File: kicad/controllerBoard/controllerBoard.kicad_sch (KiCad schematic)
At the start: 19 parts, among them J1 Conn_02x20_Top_Bottom, J2 Conn_02x20_Top_Bottom, Q1 WTM30N02VD, U1 LM3478MA

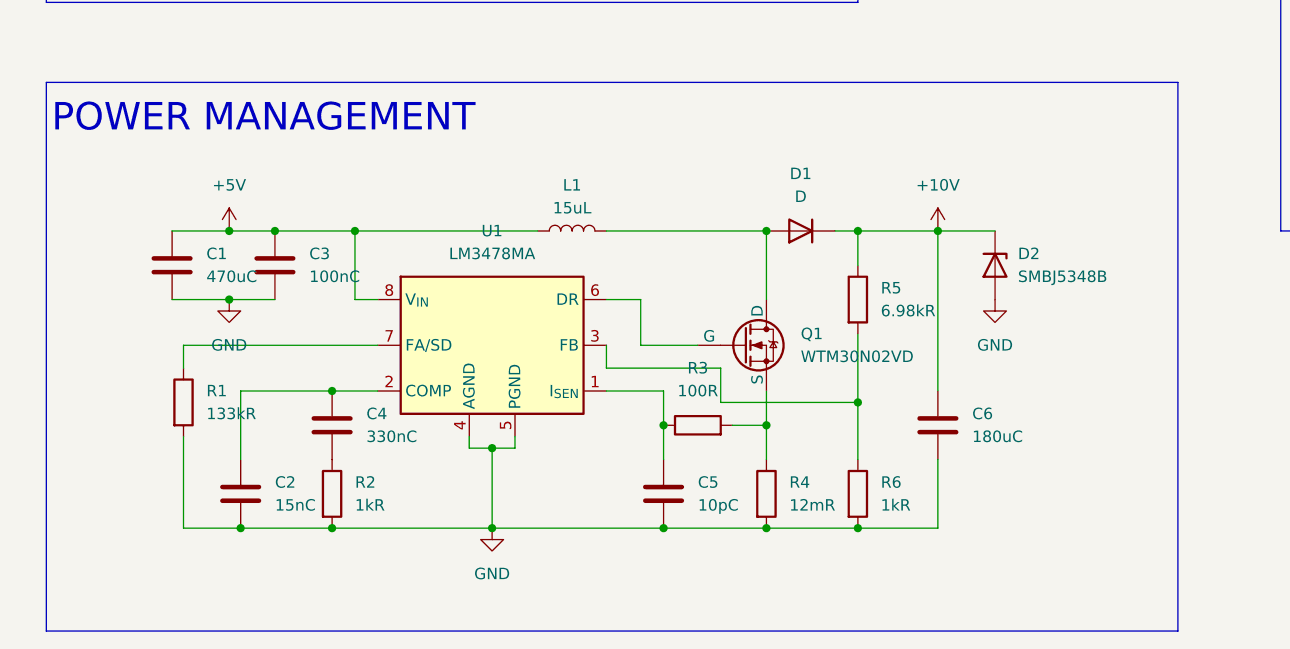
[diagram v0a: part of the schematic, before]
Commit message: change to charge pump
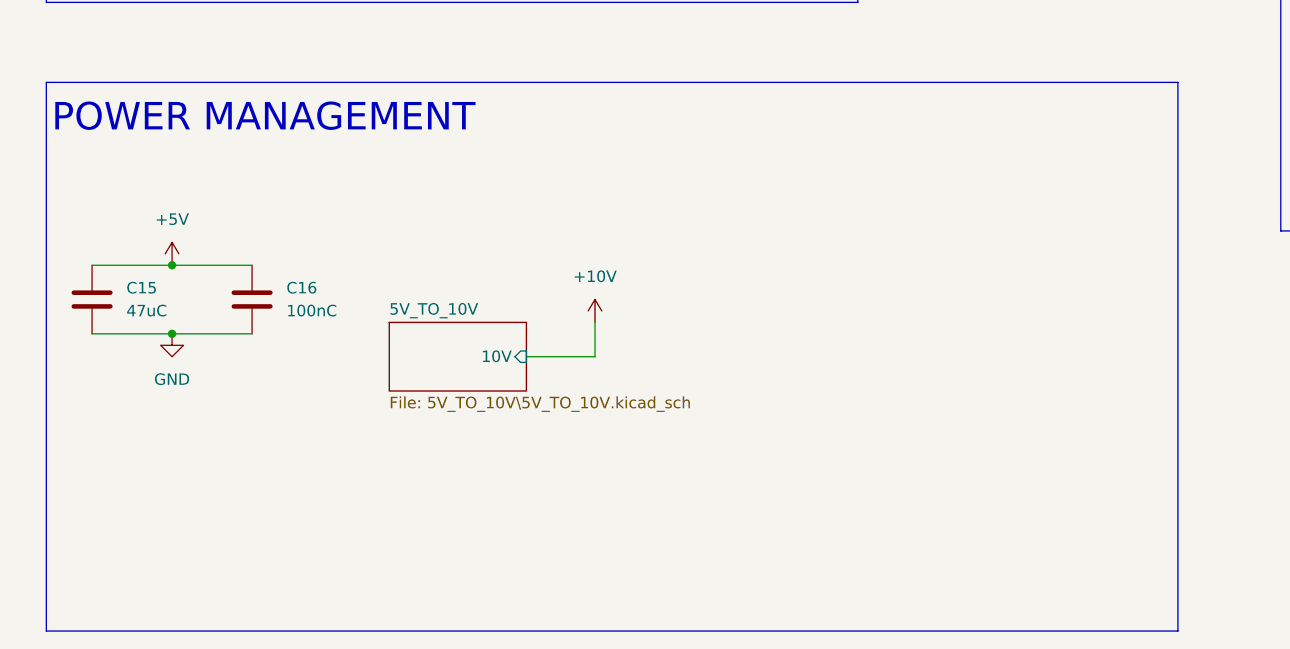
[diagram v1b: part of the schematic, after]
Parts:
- removed C1: 470uC, symbol Device:C
- removed C2: 15nC, symbol Device:C
- removed C3: 100nC, symbol Device:C
- removed C4: 330nC, symbol Device:C
- removed C5: 10pC, symbol Device:C
- removed C6: 180uC, symbol Device:C
- removed D1: D, symbol Device:D
- removed D2: SMBJ5348B, symbol Device:D_Zener
- removed L1: 15uL, symbol Device:L
- removed Q1: WTM30N02VD, symbol Simulation_SPICE:NMOS
- removed R1: 133kR, symbol Device:R
- removed R2, R6: 1kR, symbol Device:R
- removed R3: 100R, symbol Device:R
- removed R4: 12mR, symbol Device:R
- removed R5: 6.98kR, symbol Device:R
- removed U1: LM3478MA, Package_SO:SOIC-8_3.9x4.9mm_P1.27mm, symbol Regulator_Controller:LM3478MA
- added C15: 47uC, symbol Device:C
- added C16: 100nC, symbol Device:C
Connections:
- net +5V: now also C15.1, C16.1
- net GND: now also C15.2, C16.2
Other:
- added sheet 5V_TO_10V (5V_TO_10V\5V_TO_10V.kicad_sch)
